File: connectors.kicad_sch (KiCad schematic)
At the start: 10 parts, among them J3 Serial Wire Debug, J4 JST-PH, J7 USB_C_Receptacle_USB2.0, J8 External UART, J9 External I2C, U2 USBLC6-2SC6

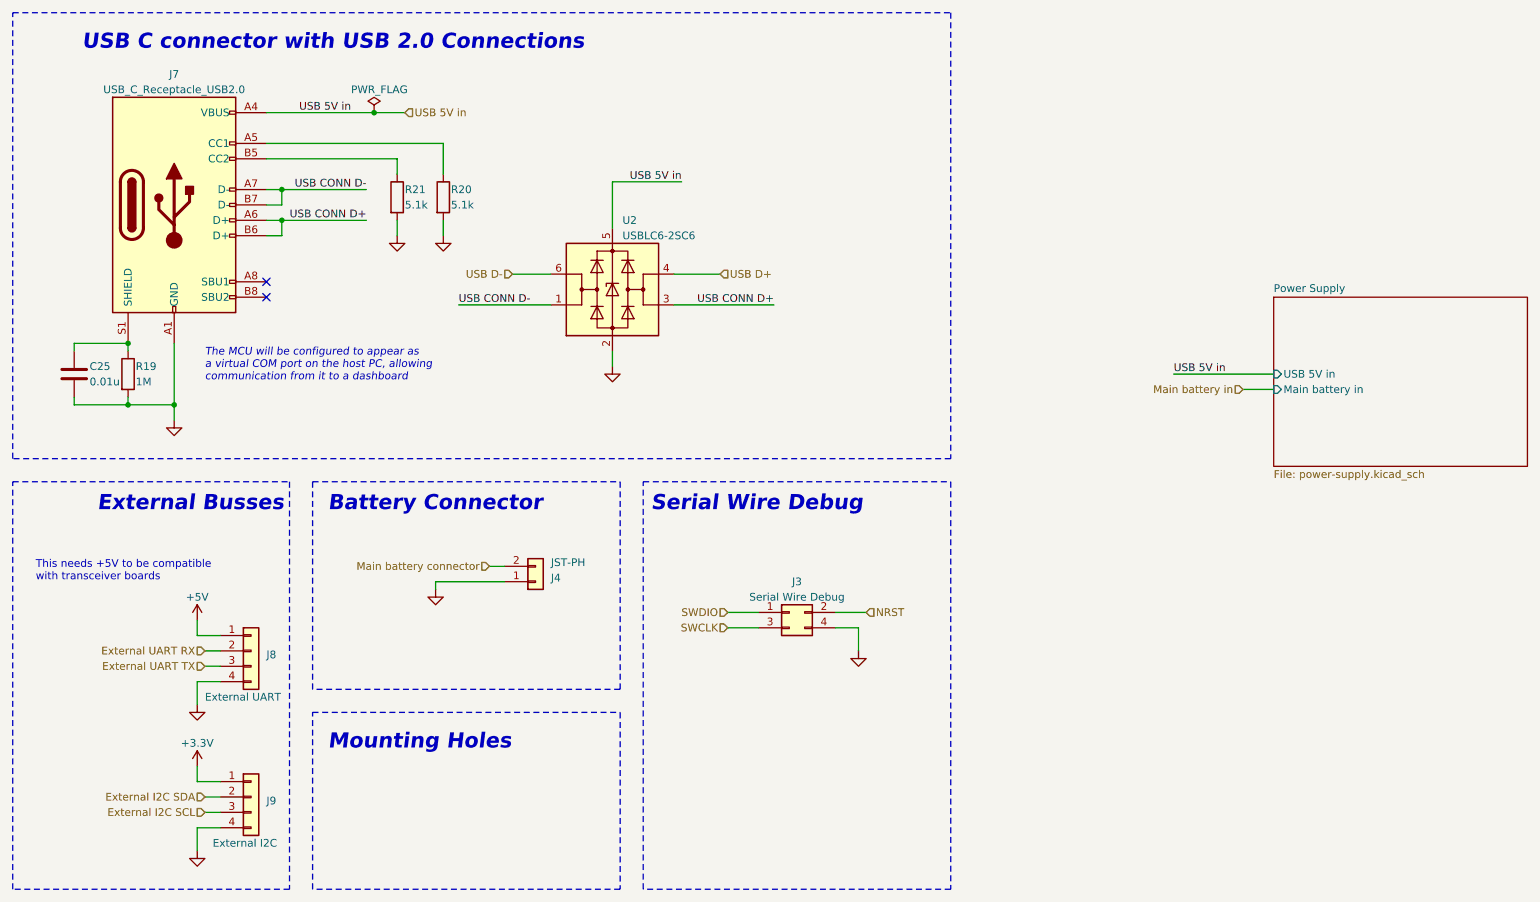
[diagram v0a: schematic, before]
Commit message: Updating with notes from Adam
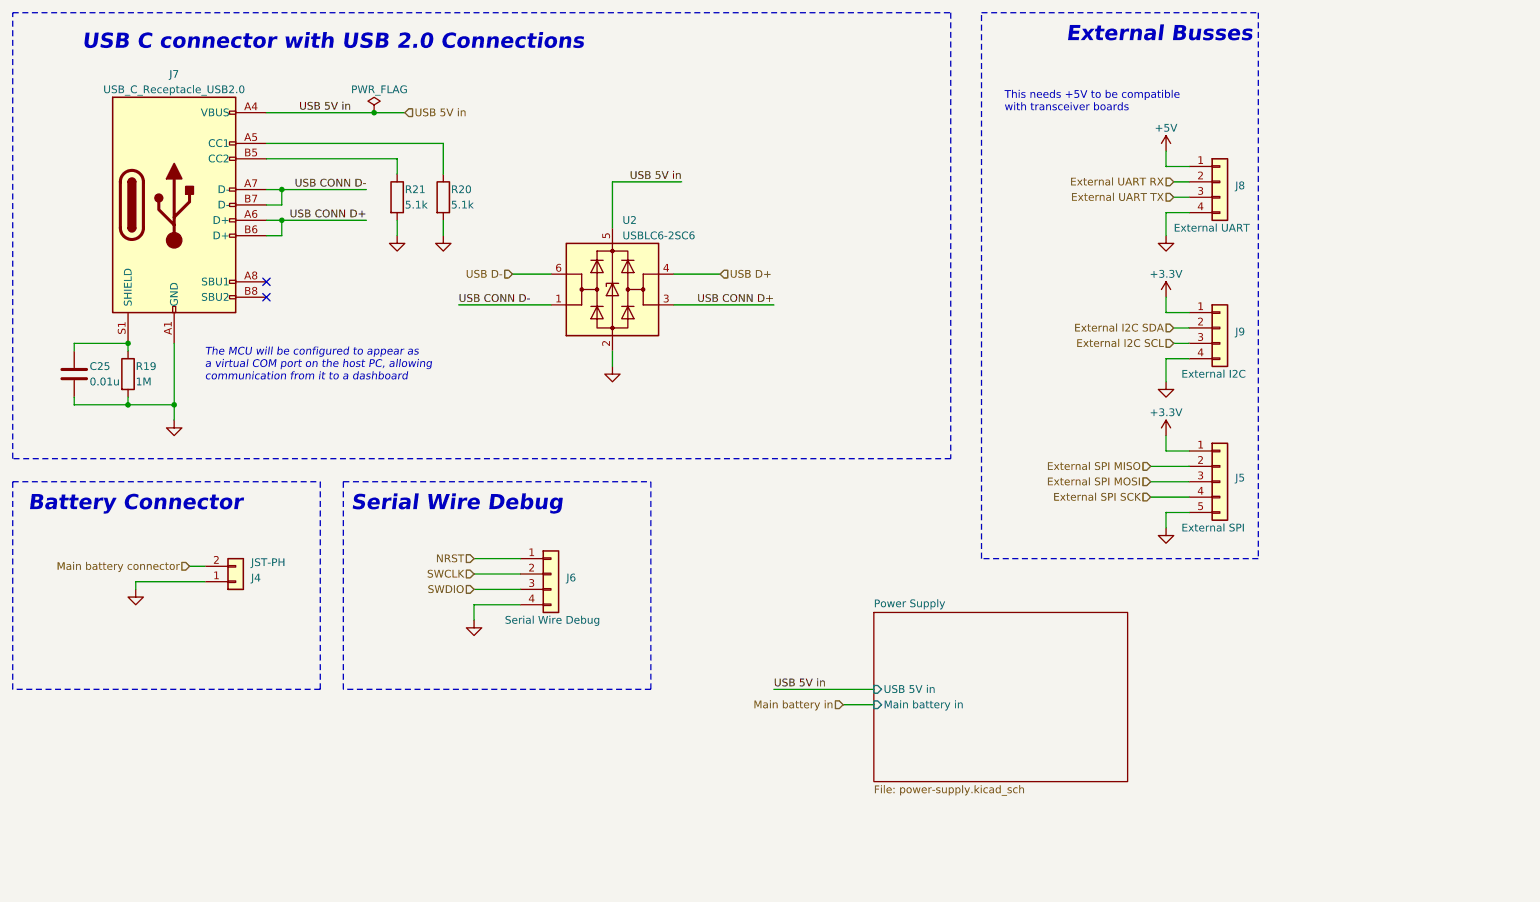
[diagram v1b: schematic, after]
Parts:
- removed J3: Serial Wire Debug, Connector_PinHeader_2.54mm:PinHeader_2x02_P2.54mm_Vertical, symbol Connector_Generic:Conn_02x02_Odd_Even
- added J5: External SPI, Connector_Molex:Molex_PicoBlade_53048-0510_1x05_P1.25mm_Horizontal, symbol Connector_Generic:Conn_01x05
- added J6: Serial Wire Debug, Connector_Molex:Molex_PicoBlade_53048-0410_1x04_P1.25mm_Horizontal, symbol Connector_Generic:Conn_01x04
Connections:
- net +3.3V: now also J5.1 (Pin_1)
- net GND: now also J5.5 (Pin_5), J6.4 (Pin_4)
- net NRST: now also J6.1 (Pin_1)
- net SWCLK: now also J6.2 (Pin_2)
- net SWDIO: now also J6.3 (Pin_3)
- new net External SPI MISO: J5.2 (Pin_2)
- new net External SPI MOSI: J5.3 (Pin_3)
- new net External SPI SCK: J5.4 (Pin_4)
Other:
- note removed: "Mounting Holes"
- moved on the sheet: J4, J8, J9

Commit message: Finished final(tm) updates for v1.1
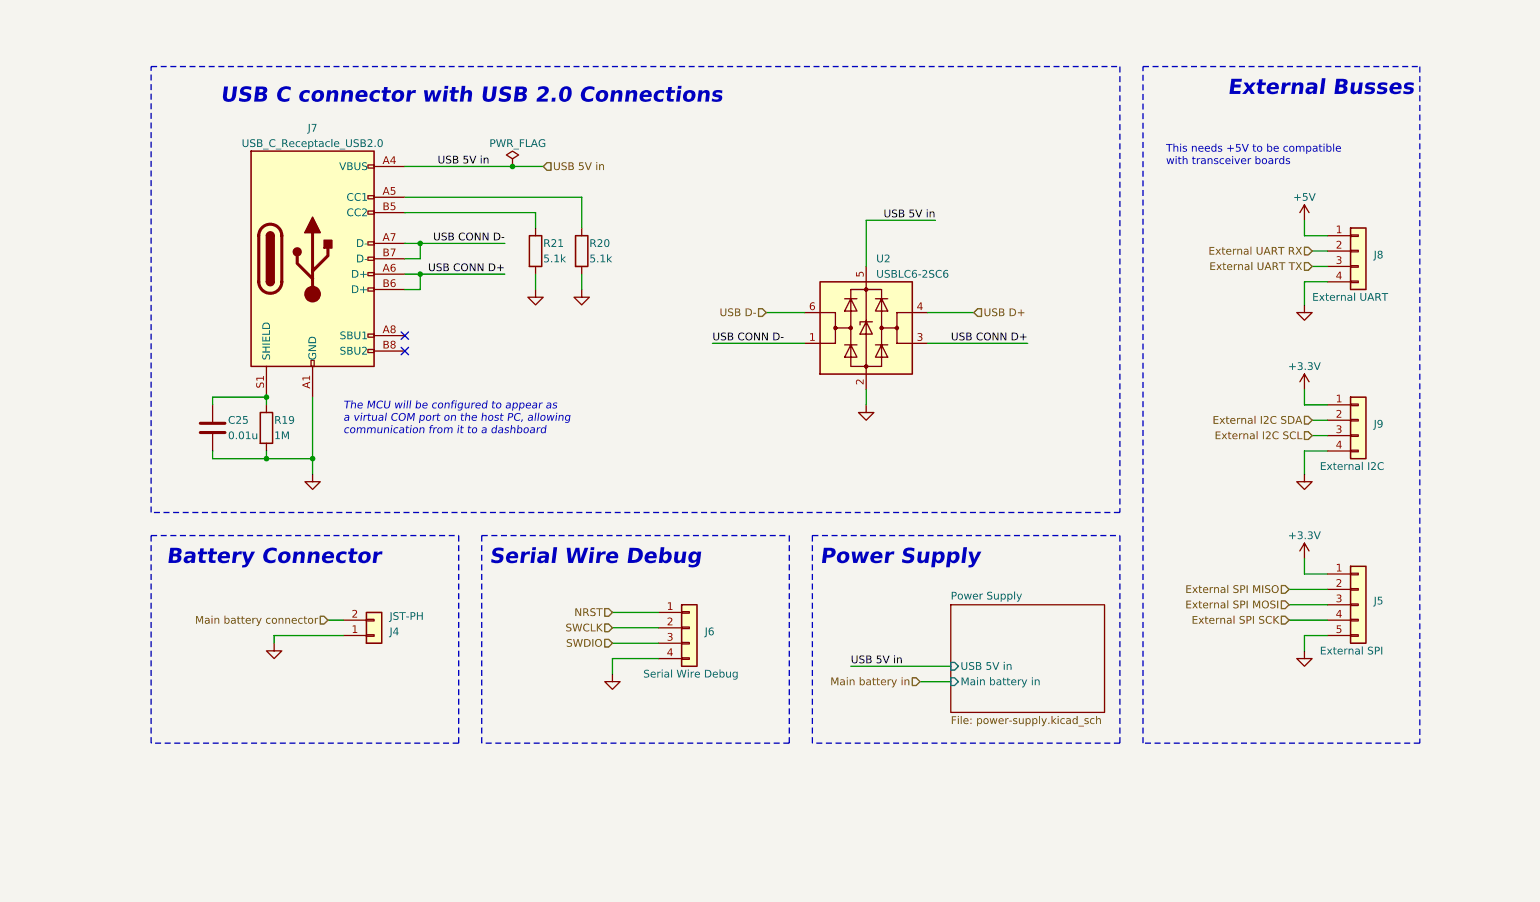
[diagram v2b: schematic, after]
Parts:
- J4: footprint Connector_JST:JST_PH_B2B-PH-K_1x02_P2.00mm_Vertical -> Connector_JST:JST_PH_S2B-PH-K_1x02_P2.00mm_Horizontal
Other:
- note added: "Power Supply"
- moved on the sheet: C25, J4, J5, J6, J7, J8, J9, R19, R20, R21, U2
